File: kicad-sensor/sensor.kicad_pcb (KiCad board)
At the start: 2 copper layers, 30 x 16 mm, 33 parts, among them J1 To main board J7, U1 BNO085, U2 BME688, U3 TSL25911FN, Y1 32.768kHz

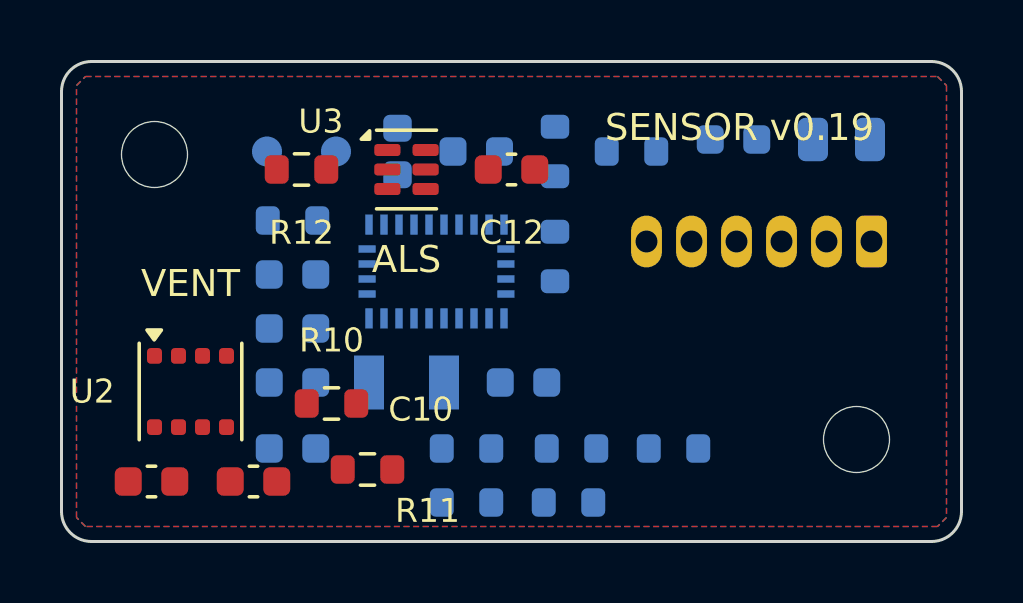
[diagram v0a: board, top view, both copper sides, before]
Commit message: manual arrangement
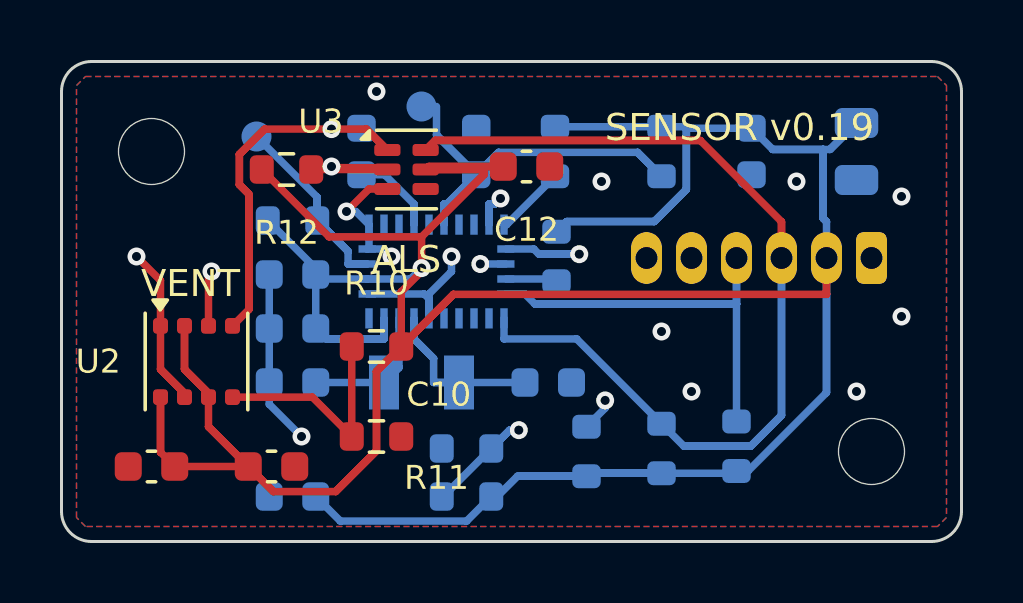
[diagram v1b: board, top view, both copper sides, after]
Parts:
- moved TP1 3.22 mm to (12.0, 1.50)
- moved R1 3.00 mm to (20.0, 12.9), turned to 90 degrees
- moved R10 2.42 mm to (10.5, 9.50)
- moved R2 2.10 mm to (22.5, 12.8), turned to 90 degrees
- moved R9 1.80 mm to (17.5, 13.0), turned to 90 degrees
- moved C5 1.60 mm to (7.70, 14.5)
- moved C6 1.20 mm to (10.0, 3.00)
- moved R11 1.14 mm to (10.5, 12.5)
- moved U2 1.02 mm to (4.50, 10.0)
- moved R6 1.00 mm to (20.0, 3.00), turned to -90 degrees
- moved C8 0.83 mm to (16.2, 10.7)
- moved C10 0.78 mm to (7.00, 13.5)
- moved C2 0.72 mm to (23.0, 3.00), turned to -90 degrees
- moved H2 0.64 mm to (27.0, 13.0)
- moved C1 0.64 mm to (26.5, 3.00), turned to -90 degrees
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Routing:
- net +3V3: track 0.00 -> 157.8 mm, vias 0 -> 1
- net I2C_SDA: track 0.00 -> 73.4 mm, vias 0 -> 1
- net I2C_SCL: track 0.00 -> 62.9 mm, vias 0 -> 1
- net GND: track 0.00 -> 41.8 mm, vias 0 -> 13
- net ALS_INT: track 0.00 -> 26.4 mm, vias 0 -> 1
- net BNO_NRST: track 0.00 -> 18.0 mm
- net BNO_ENV_SDA: track 0.00 -> 14.5 mm, vias 0 -> 2
- net SENSOR_INT: track 0.00 -> 12.2 mm, vias 0 -> 1
- net BNO_SA0: track 0.00 -> 11.6 mm, vias 0 -> 2
- net BNO_BOOTN: track 0.00 -> 9.01 mm
- net Net-(U1-XOUT32/CLKSEL1): track 0.00 -> 7.91 mm
- net Net-(U2-SDO): track 0.00 -> 7.52 mm
- net Net-(U1-XIN32): track 0.00 -> 5.33 mm
- net Net-(U1-CAP): track 0.00 -> 3.02 mm
- net BNO_ENV_SCL: track 0.00 -> 2.46 mm
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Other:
- copper layers 2 -> 4
